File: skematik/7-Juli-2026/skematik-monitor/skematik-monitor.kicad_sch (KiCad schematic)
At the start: 11 parts, among them K1 FOTEK SSR, M1 Motor_AC, U1 ESP32-DevKitC, U2 DS18B20, U3 ACS712xLCTR-05B, U4 ADXL345, U5 A3104xLH

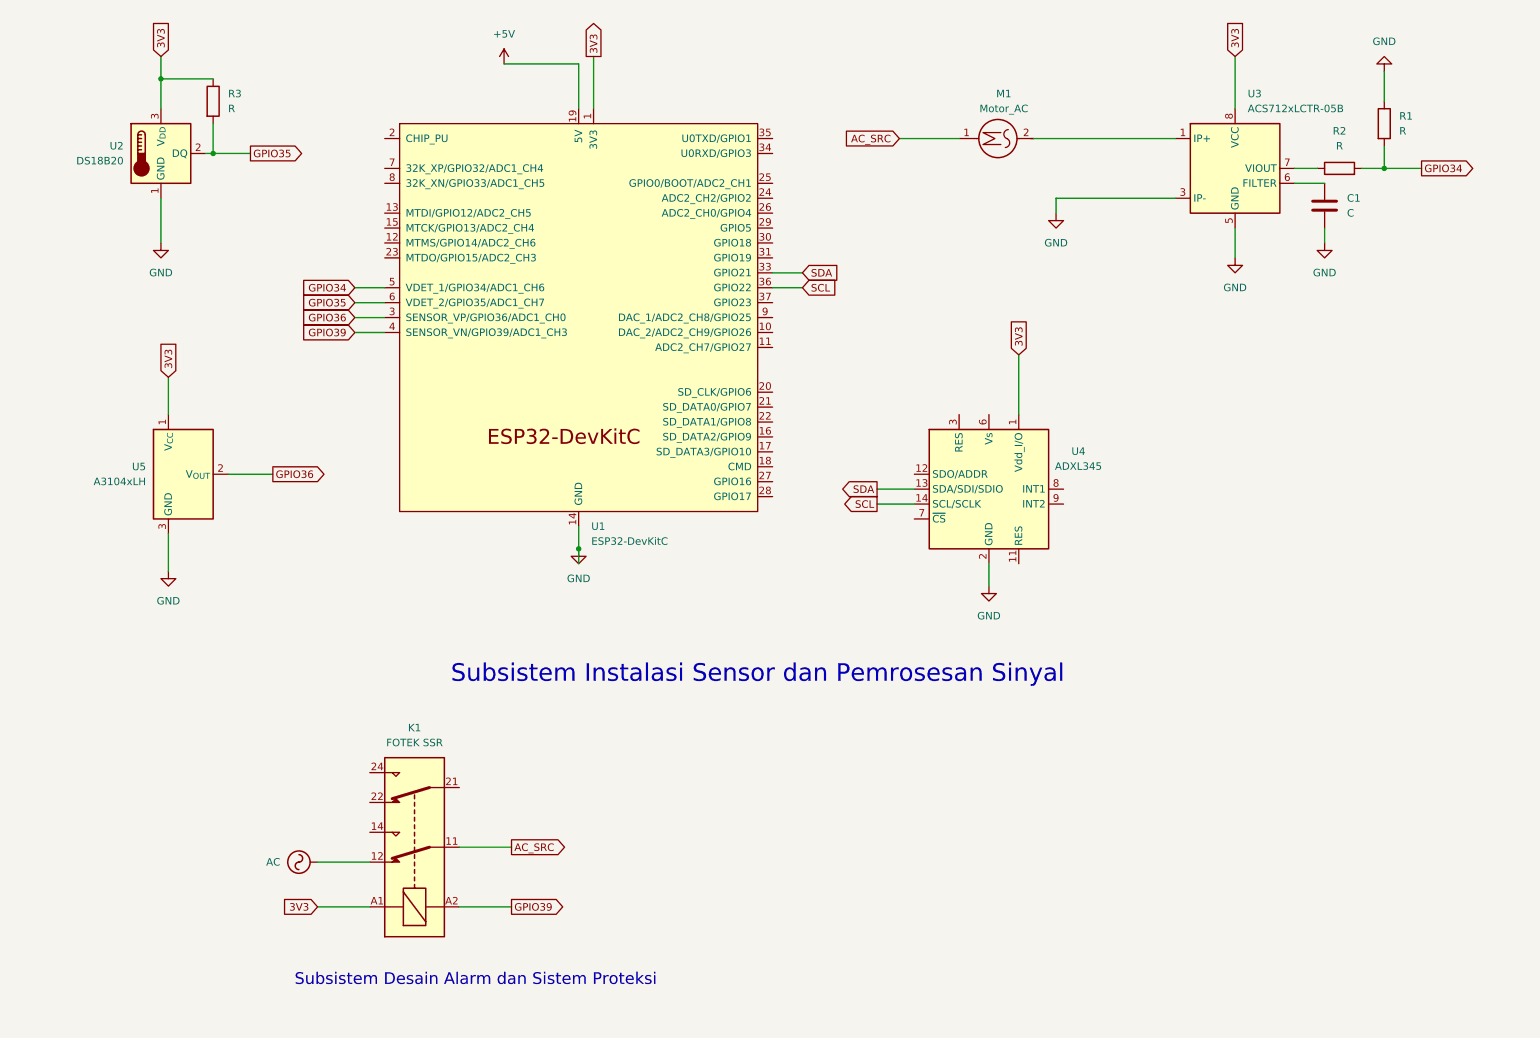
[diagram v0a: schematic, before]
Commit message: 03-08-2026 updates
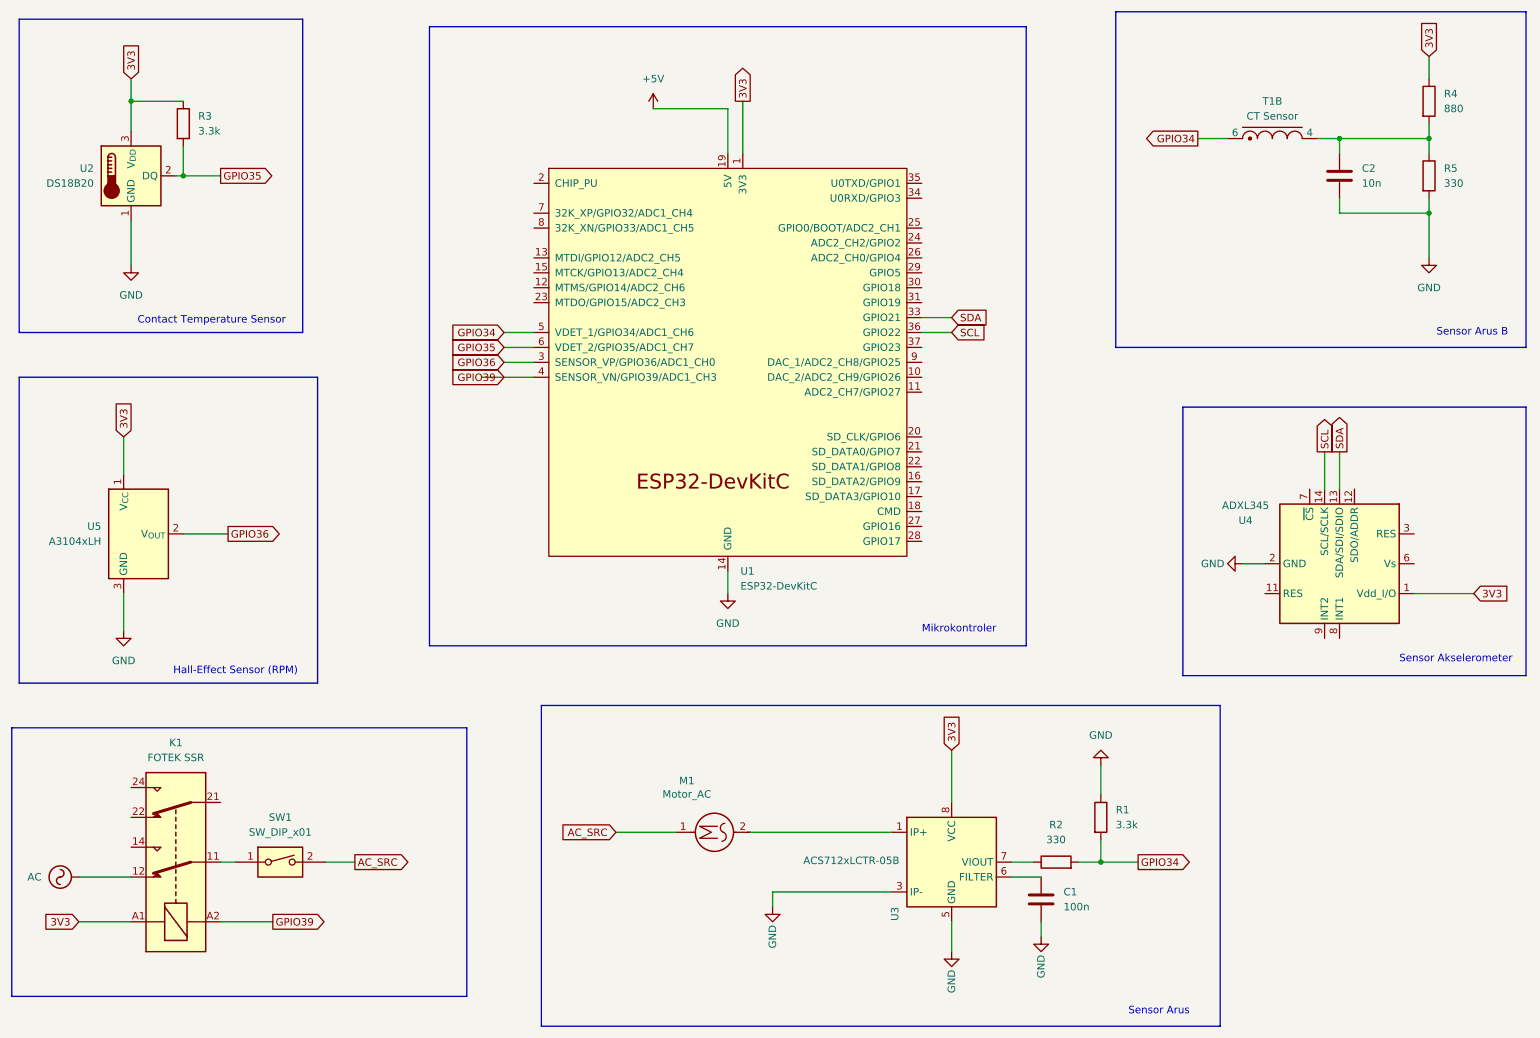
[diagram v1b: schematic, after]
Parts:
- added C2: 10n, Capacitor_THT:CP_Radial_D7.5mm_P2.50mm, symbol Device:C
- added R4: 880, Resistor_THT:R_Axial_DIN0204_L3.6mm_D1.6mm_P2.54mm_Vertical, symbol Device:R
- added R5: 330, Resistor_THT:R_Axial_DIN0204_L3.6mm_D1.6mm_P2.54mm_Vertical, symbol Device:R
- added SW1: SW_DIP_x01, symbol Switch:SW_DIP_x01
- added T1: CT Sensor, Transformer_SMD:Transformer_Coilcraft_CST1, symbol Transformer:CST1_Split
- C1: value C -> 100n; footprint (none) -> Capacitor_THT:CP_Axial_L10.0mm_D6.0mm_P15.00mm_Horizontal
- R1, R3: value R -> 3.3k; footprint (none) -> Resistor_THT:R_Axial_DIN0204_L3.6mm_D1.6mm_P2.54mm_Vertical
- R2: value R -> 330; footprint (none) -> Resistor_THT:R_Axial_DIN0204_L3.6mm_D1.6mm_P2.54mm_Vertical
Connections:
- net 3V3: now also R4.1
- net AC_SRC: now also SW1.2; no longer K1.11
- net GND: now also C2.2, R5.2
- net GPIO34: now also T1.6
- new net: C2.1, R4.2, R5.1, T1.4
- new net: K1.11, SW1.1
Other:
- note added: "Contact Temperature Sensor"
- note added: "Hall-Effect Sensor (RPM)"
- note added: "Mikrokontroler"
- note added: "Sensor Akselerometer"
- note added: "Sensor Arus"
- note added: "Sensor Arus B"
- note removed: "Subsistem Desain Alarm dan Sistem Proteksi"
- note removed: "Subsistem Instalasi Sensor dan Pemrosesan Sinyal"
- moved on the sheet: C1, K1, M1, R1, R2, R3, U1, U2, U3, U4, U5
